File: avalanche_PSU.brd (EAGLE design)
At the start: 59.7 x 22.5 mm, 15 parts

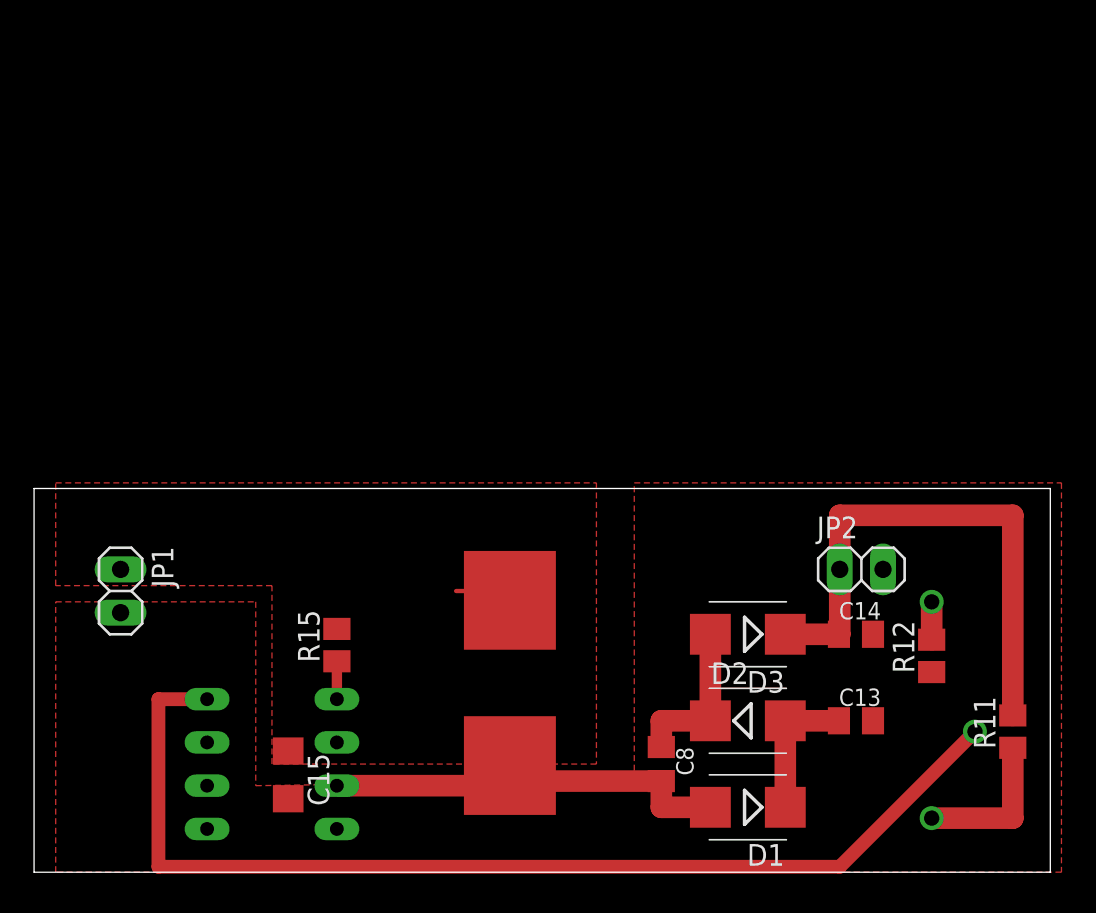
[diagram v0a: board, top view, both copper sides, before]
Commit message: altered artwork
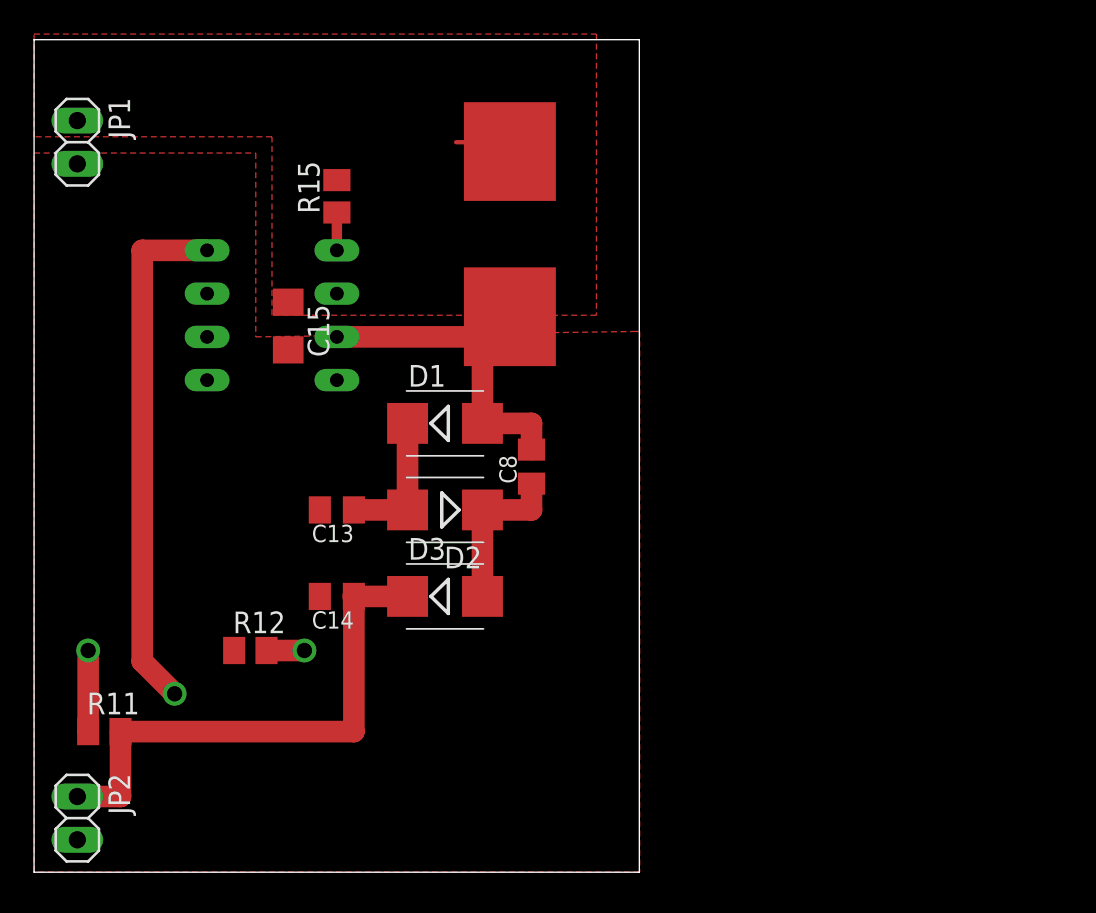
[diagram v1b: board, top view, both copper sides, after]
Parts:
- moved R11 53.3 mm to (4.13, 8.26), turned to 0 degrees
- moved JP2 48.3 mm to (2.54, 3.17), turned to 270 degrees
- moved R13 45.9 mm to (8.26, 11.7), turned to 0 degrees
- moved R12 40.0 mm to (12.7, 13.0), turned to 0 degrees
- moved C13 32.9 mm to (17.8, 21.3), turned to 180 degrees
- moved C14 30.6 mm to (17.8, 16.2), turned to 180 degrees
- moved D1 28.7 mm to (24.1, 26.4), turned to 0 degrees
- moved JP1 26.5 mm to (2.54, 42.9)
- moved C15 26.4 mm to (14.9, 32.1)
- moved L1 26.4 mm to (27.9, 37.5)
- moved R15 26.4 mm to (17.8, 39.7)
- moved U$3 26.4 mm to (14.0, 32.7)
- moved D2 21.7 mm to (24.1, 21.3), turned to 180 degrees
- moved C8 19.1 mm to (29.2, 23.8), turned to 90 degrees
- moved D3 17.9 mm to (24.1, 16.2), turned to 0 degrees
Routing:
- net N$40: track 63.9 -> 30.6 mm
- net N$39: track 8.89 -> 4.76 mm
- net N$37: track 24.9 -> 21.7 mm
- net N$25: track 32.1 -> 31.2 mm
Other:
- board size 59.7 x 22.5 mm -> 35.5 x 48.9 mm
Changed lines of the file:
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@@
 <board>
 <plain>
-<wire x1="0" y1="0" x2="59.67" y2="0" width="0" layer="20"/>
-<wire x1="59.67" y1="0" x2="59.67" y2="22.53" width="0" layer="20"/>
-<wire x1="59.67" y1="22.53" x2="0" y2="22.53" width="0" layer="20"/>
-<wire x1="0" y1="22.53" x2="0" y2="0" width="0" layer="20"/>
+<wire x1="0" y1="0" x2="35.54" y2="0" width="0" layer="20"/>
+<wire x1="35.54" y1="0" x2="35.54" y2="48.8825" width="0" layer="20"/>
+<wire x1="35.54" y1="48.8825" x2="0" y2="48.8825" width="0" layer="20"/>
+<wire x1="0" y1="48.8825" x2="0" y2="0" width="0" layer="20"/>
 </plain>
 <attributes>
@@
 </autorouter>
 <elements>
-<element name="U$3" library="LT1073" package="DIL08" value="LT1073" x="13.97" y="6.35" rot="MR270"/>
-<element name="D1" library="diode" package="SMB" value="ES2D" x="41.91" y="3.81" rot="R180"/>
-<element name="D2" library="diode" package="SMB" value="ES2D" x="41.91" y="8.89"/>
-<element name="D3" library="diode" package="SMB" value="ES2D" x="41.91" y="13.97" rot="R180"/>
-<element name="R11" library="resistor" package="M0805" value="1M" x="57.4675" y="8.255" rot="R90"/>
-<element name="R12" library="resistor" package="M0805" value="2k4" x="52.705" y="12.7" rot="R90"/>
-<element name="R13" library="resistor" package="RTRIMT18" value="10k" x="53.975" y="8.255" rot="MR270"/>
-<element name="R15" library="resistor" package="M0805" value="220" x="17.78" y="13.335" rot="R90"/>
-<element name="C15" library="resistor" package="C1206" value="" x="14.9225" y="5.715" rot="R270"/>
-<element name="C8" library="resistor" package="C0805K" value="" x="36.83" y="6.35" rot="R270"/>
-<element name="C13" library="resistor" package="C0805K" value="" x="48.26" y="8.89"/>
-<element name="C14" library="resistor" package="C0805K" value="" x="48.26" y="13.97"/>
-<element name="L1" library="SRR1280" package="SRR1280" value="" x="27.94" y="11.1125" rot="R270"/>
-<element name="JP1" library="pinhead" package="1X02" value="" x="5.08" y="16.51" rot="R270"/>
-<element name="JP2" library="pinhead" package="1X02" value="" x="48.5775" y="17.78"/>
+<element name="U$3" library="LT1073" package="DIL08" value="LT1073" x="13.97" y="32.7025" rot="MR270"/>
+<element name="D1" library="diode" package="SMB" value="ES2D" x="24.13" y="26.3525"/>
+<element name="D2" library="diode" package="SMB" value="ES2D" x="24.13" y="21.2725" rot="R180"/>
+<element name="D3" library="diode" package="SMB" value="ES2D" x="24.13" y="16.1925"/>
+<element name="R11" library="resistor" package="M0805" value="1M" x="4.1275" y="8.255"/>
+<element name="R12" library="resistor" package="M0805" value="2k4" x="12.7" y="13.0175"/>
+<element name="R13" library="resistor" package="RTRIMT18" value="10k" x="8.255" y="11.7475" rot="MR0"/>
+<element name="R15" library="resistor" package="M0805" value="220" x="17.78" y="39.6875" rot="R90"/>
+<element name="C15" library="resistor" package="C1206" value="" x="14.9225" y="32.0675" rot="R270"/>
+<element name="C8" library="resistor" package="C0805K" value="" x="29.21" y="23.8125" rot="R90"/>
+<element name="C13" library="resistor" package="C0805K" value="" x="17.78" y="21.2725" rot="R180"/>
+<element name="C14" library="resistor" package="C0805K" value="" x="17.78" y="16.1925" rot="R180"/>
+<element name="L1" library="SRR1280" package="SRR1280" value="" x="27.94" y="37.465" rot="R270"/>
+<element name="JP1" library="pinhead" package="1X02" value="" x="2.54" y="42.8625" rot="R270"/>
+<element name="JP2" library="pinhead" package="1X02" value="" x="2.54" y="3.175" rot="R270"/>
 </elements>
 <signals>
@@
 <contactref element="JP1" pad="2"/>
 <contactref element="JP2" pad="2"/>
-<polygon width="0.4064" layer="1" isolate="0.3048">
-<vertex x="1.27" y="15.875"/>
-<vertex x="13.0175" y="15.875"/>
-<vertex x="13.0175" y="5.08"/>
-<vertex x="35.2425" y="5.3975"/>
-<vertex x="35.2425" y="22.86"/>
-<vertex x="60.325" y="22.86"/>
-<vertex x="60.325" y="0"/>
-<vertex x="1.27" y="0"/>
+<polygon width="0.4064" layer="1" isolate="0.4064">
+<vertex x="0" y="42.2275"/>
+<vertex x="13.0175" y="42.2275"/>
+<vertex x="13.0175" y="31.4325"/>
+<vertex x="35.2425" y="31.75"/>
+<vertex x="35.56" y="31.75"/>
+<vertex x="35.56" y="0"/>
+<vertex x="0" y="0"/>
 </polygon>
 </signal>
@@
 <contactref element="JP1" pad="1"/>
 <polygon width="0.4064" layer="1" isolate="0.3048" thermals="no">
-<vertex x="1.27" y="22.86"/>
-<vertex x="33.02" y="22.86"/>
-<vertex x="33.02" y="6.35"/>
-<vertex x="13.97" y="6.35"/>
-<vertex x="13.97" y="16.8275"/>
-<vertex x="1.27" y="16.8275"/>
+<vertex x="0" y="49.2125"/>
+<vertex x="33.02" y="49.2125"/>
+<vertex x="33.02" y="32.7025"/>
+<vertex x="13.97" y="32.7025"/>
+<vertex x="13.97" y="43.18"/>
+<vertex x="0" y="43.18"/>
 </polygon>
-<wire x1="24.7828" y1="16.51" x2="27.94" y2="16.51" width="0.254" layer="1"/>
-<wire x1="27.94" y1="16.51" x2="27.94" y2="15.9625" width="0.254" layer="1"/>
+<wire x1="24.7828" y1="42.8625" x2="27.94" y2="42.8625" width="0.254" layer="1"/>
+<wire x1="27.94" y1="42.8625" x2="27.94" y2="42.315" width="0.254" layer="1"/>
 </signal>
 <signal name="N$13">
@@
 <contactref element="D2" pad="A"/>
 <contactref element="C13" pad="1"/>
-<wire x1="44.11" y1="3.81" x2="44.11" y2="8.89" width="1.27" layer="1"/>
-<wire x1="44.11" y1="8.89" x2="47.26" y2="8.89" width="1.27" layer="1"/>
+<wire x1="21.93" y1="26.3525" x2="21.93" y2="21.2725" width="1.27" layer="1"/>
+<wire x1="21.93" y1="21.2725" x2="18.78" y2="21.2725" width="1.27" layer="1"/>
 </signal>
 <signal name="N$24">
@@
 <contactref element="D2" pad="C"/>
 <contactref element="C8" pad="1"/>
-<wire x1="39.71" y1="8.89" x2="36.83" y2="8.89" width="1.27" layer="1"/>
-<wire x1="36.83" y1="8.89" x2="36.83" y2="7.35" width="1.27" layer="1"/>
-<wire x1="39.71" y1="13.97" x2="39.71" y2="8.89" width="1.27" layer="1"/>
+<wire x1="26.33" y1="21.2725" x2="29.21" y2="21.2725" width="1.27" layer="1"/>
+<wire x1="29.21" y1="21.2725" x2="29.21" y2="22.8125" width="1.27" layer="1"/>
+<wire x1="26.33" y1="16.1925" x2="26.33" y2="21.2725" width="1.27" layer="1"/>
 </signal>
 <signal name="N$25">
@@
 <contactref element="C14" pad="1"/>
 <contactref element="JP2" pad="1"/>
-<wire x1="47.26" y1="13.97" x2="44.11" y2="13.97" width="1.27" layer="1"/>
-<wire x1="47.26" y1="13.97" x2="47.3075" y2="13.97" width="1.27" layer="1"/>
-<wire x1="47.3075" y1="13.97" x2="47.3075" y2="17.78" width="1.27" layer="1"/>
-<wire x1="57.4675" y1="9.205" x2="57.4675" y2="20.955" width="1.27" layer="1"/>
-<wire x1="57.4675" y1="20.955" x2="47.3075" y2="20.955" width="1.27" layer="1"/>
-<wire x1="47.3075" y1="20.955" x2="47.3075" y2="17.78" width="1.27" layer="1"/>
+<wire x1="18.78" y1="16.1925" x2="21.93" y2="16.1925" width="1.27" layer="1"/>
+<wire x1="18.78" y1="16.1925" x2="18.7325" y2="16.1925" width="1.27" layer="1"/>
+<wire x1="5.0775" y1="8.255" x2="18.78" y2="8.255" width="1.27" layer="1"/>
+<wire x1="18.78" y1="8.255" x2="18.78" y2="16.1925" width="1.27" layer="1"/>
+<wire x1="2.54" y1="4.445" x2="5.0775" y2="4.445" width="1.27" layer="1"/>
+<wire x1="5.0775" y1="4.445" x2="5.0775" y2="8.255" width="1.27" layer="1"/>
 </signal>
 <signal name="N$37">
@@
 <contactref element="C8" pad="2"/>
 <contactref element="L1" pad="P$2"/>
-<wire x1="17.78" y1="5.08" x2="27.94" y2="5.08" width="1.27" layer="1"/>
-<wire x1="36.83" y1="5.35" x2="28.575" y2="5.35" width="1.27" layer="1"/>
-<wire x1="28.575" y1="5.35" x2="28.575" y2="5.08" width="1.27" layer="1"/>
-<wire x1="28.575" y1="5.08" x2="27.94" y2="5.08" width="1.27" layer="1"/>
-<wire x1="27.94" y1="5.08" x2="27.94" y2="6.2625" width="1.27" layer="1"/>
-<wire x1="39.71" y1="3.81" x2="36.83" y2="3.81" width="1.27" layer="1"/>
-<wire x1="36.83" y1="3.81" x2="36.83" y2="5.35" width="1.27" layer="1"/>
+<wire x1="17.78" y1="31.4325" x2="26.33" y2="31.4325" width="1.27" layer="1"/>
+<wire x1="28.575" y1="31.7025" x2="28.575" y2="31.4325" width="1.27" layer="1"/>
+<wire x1="28.575" y1="31.4325" x2="27.94" y2="31.4325" width="1.27" layer="1"/>
+<wire x1="27.94" y1="31.4325" x2="27.94" y2="32.615" width="1.27" layer="1"/>
+<wire x1="26.33" y1="26.3525" x2="29.21" y2="26.3525" width="1.27" layer="1"/>
+<wire x1="29.21" y1="26.3525" x2="29.21" y2="24.8125" width="1.27" layer="1"/>
+<wire x1="27.94" y1="31.4325" x2="26.33" y2="31.4325" width="1.27" layer="1"/>
+<wire x1="26.33" y1="31.4325" x2="26.33" y2="26.3525" width="1.27" layer="1"/>
 </signal>
 <signal name="N$38">
 <contactref element="R13" pad="1"/>
 <contactref element="R12" pad="2"/>
-<wire x1="52.705" y1="13.65" x2="52.705" y2="15.875" width="1.27" layer="1"/>
+<wire x1="15.875" y1="13.0175" x2="13.65" y2="13.0175" width="1.27" layer="1"/>
 </signal>
 <signal name="N$39">
 <contactref element="R13" pad="3"/>
 <contactref element="R11" pad="1"/>
-<wire x1="52.705" y1="3.175" x2="57.4675" y2="3.175" width="1.27" layer="1"/>
-<wire x1="57.4675" y1="3.175" x2="57.4675" y2="7.305" width="1.27" layer="1"/>
+<wire x1="3.1775" y1="8.255" x2="3.175" y2="8.255" width="1.27" layer="1"/>
+<wire x1="3.175" y1="8.255" x2="3.175" y2="13.0175" width="1.27" layer="1"/>
 </signal>
 <signal name="N$40">
 <contactref element="U$3" pad="8"/>
 <contactref element="R13" pad="2"/>
-<wire x1="55.245" y1="8.255" x2="47.3075" y2="0.3175" width="0.8128" layer="1"/>
-<wire x1="47.3075" y1="0.3175" x2="7.3025" y2="0.3175" width="0.8128" layer="1"/>
-<wire x1="7.3025" y1="0.3175" x2="7.3025" y2="10.16" width="0.8128" layer="1"/>
-<wire x1="7.3025" y1="10.16" x2="10.16" y2="10.16" width="0.8128" layer="1"/>
+<wire x1="8.255" y1="10.4775" x2="6.35" y2="12.3825" width="1.27" layer="1"/>
+<wire x1="6.35" y1="12.3825" x2="6.35" y2="36.5125" width="1.27" layer="1"/>
+<wire x1="6.35" y1="36.5125" x2="10.16" y2="36.5125" width="1.27" layer="1"/>
 </signal>
 <signal name="N$41">
 <contactref element="U$3" pad="1"/>
 <contactref element="R15" pad="1"/>
-<wire x1="17.78" y1="10.16" x2="17.78" y2="12.385" width="0.6096" layer="1"/>
+<wire x1="17.78" y1="36.5125" x2="17.78" y2="38.7375" width="0.6096" layer="1"/>
 </signal>
 </signals>
